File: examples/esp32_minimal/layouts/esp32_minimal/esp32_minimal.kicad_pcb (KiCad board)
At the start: 2 copper layers, 36.2 x 26.8 mm, 20 parts

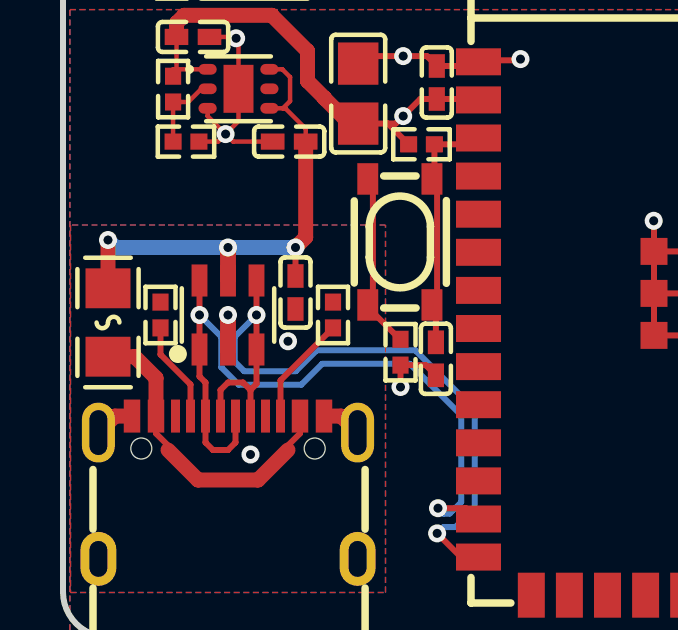
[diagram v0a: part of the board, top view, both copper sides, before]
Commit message: layout updates
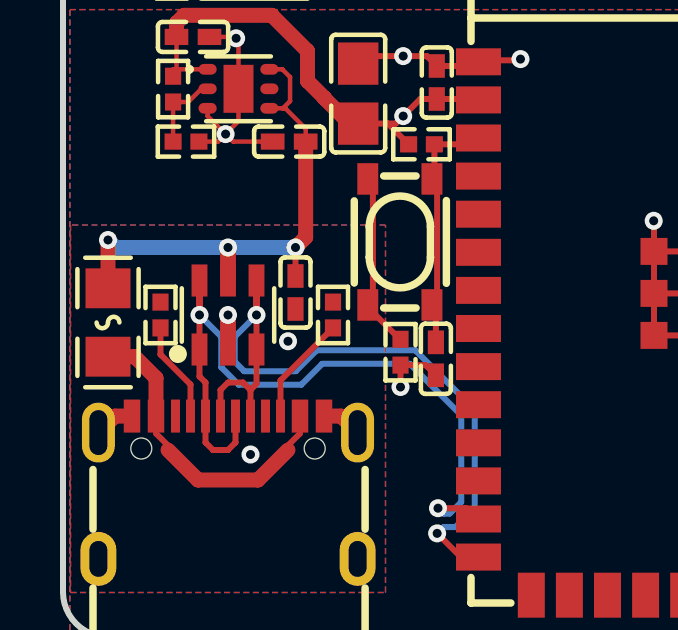
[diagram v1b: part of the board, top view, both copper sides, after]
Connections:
- net i2c[0]-SCL renamed gpios[1]-SCL
- net power-VCC renamed power_shim-VCC
- net uart[0]-SDA renamed spi[3]-SDA
- USB1 pad : net -> (no net)
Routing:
- net USB_D_P: track 24.2 -> 25.4 mm
- net USB_D_N: track 24.1 -> 25.3 mm

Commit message: lock net names with latest
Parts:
- C9: value 22µF ±20% 25V X5R -> 22µF ±20% 6.3V X5R; footprint Samsung_Electro_Mechanics_CL21A226MAQNNNE:C0805 -> Samsung_Electro_Mechanics_CL21A226MQQNNNE:C0805
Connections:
- net MOSI renamed spi[2]-MOSI
- net enable-output renamed output-output
- net gpios[10]-line renamed spi_cs[2]-line
- net gpios[12]-SCLK renamed SCLK
- net gpios[14]-SCL renamed spi_cs[3]-SCL
- net gpios[16]-SCLK renamed CTS
- net gpios[1]-SCL renamed i2c[0]-SCL
- net gpios[2]-SCK renamed i2s[0]-SCK
- net gpios[3]-WS renamed i2s[0]-WS
- net gpios[4]-SD renamed i2s[0]-SD
- net gpios[5]-SCK renamed i2s[1]-SCK
- net gpios[6]-WS renamed i2s[1]-WS
- net gpios[7]-SDA renamed SDA
- net power_shim-VCC renamed power-VCC
- net spi[3]-MISO renamed uart[1]-MISO
- net spi[3]-SDA renamed uart[0]-MOSI
- USB1 pad : (no net) -> net
